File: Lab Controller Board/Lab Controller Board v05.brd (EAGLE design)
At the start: 50 x 50 mm, 52 parts, among them Q2 NPN - 2N5088, Q3 MOSFET-NCHANNELFQP30N06L, Q4 NPN - 2N5088, Q5 MOSFET-NCHANNELFQP30N06L, Q6 NPN - 2N5088, Q7 MOSFET-NCHANNELFQP30N06L, Q8 NPN - 2N5088, U1 ATMEGA328P_TQFP, U2 CH340G, Y1 16MHZ

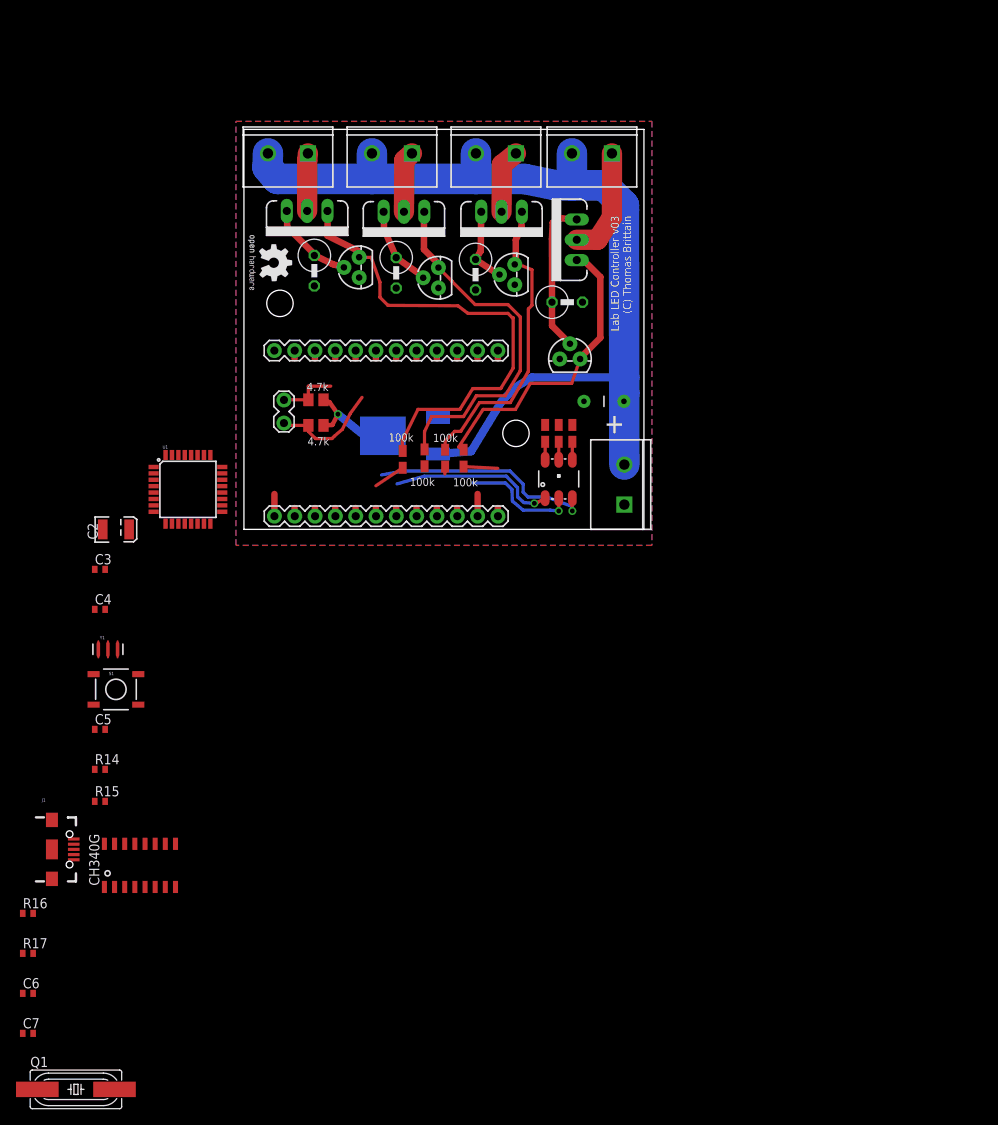
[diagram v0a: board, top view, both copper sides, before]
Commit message: Working on Lab LED
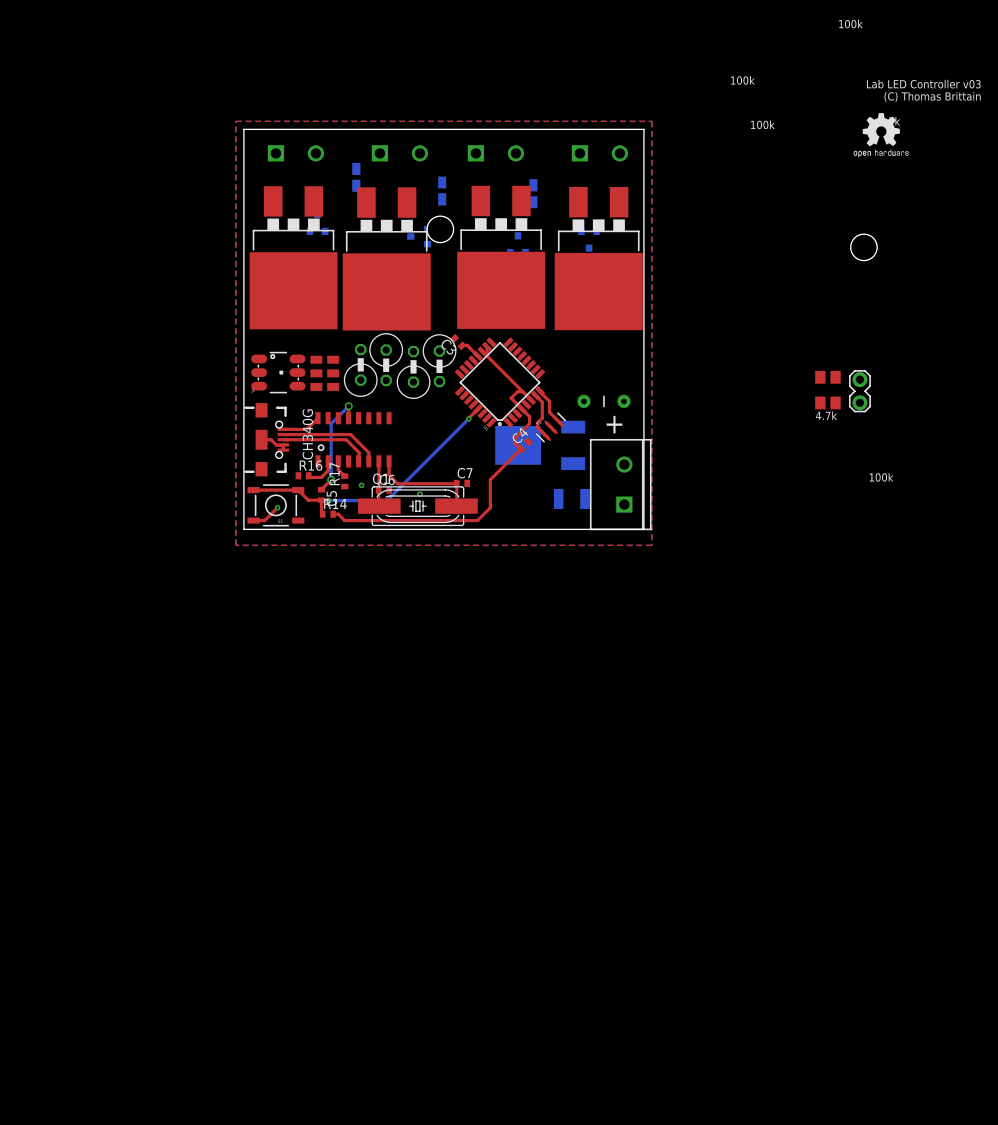
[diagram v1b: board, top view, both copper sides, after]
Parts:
- removed JP6, JP7: (no value), SparkFun-Connectors:1X12
- removed R15: 330, resistor:R0402
- FQP30N06L, Q3, Q5, Q7: value MOSFET-NCHANNELFQP30N06L -> 100A/100V; device SparkFun-DiscreteSemi:TO220V -> SparkFun-DiscreteSemi:TO-263/D2PAK
- Q2, Q4, Q6, Q8: value NPN - 2N5088 -> MMBT5088; device SparkFun-DiscreteSemi:TO-92 -> SparkFun-DiscreteSemi:SOT23-3
- moved C7 87.6 mm to (27.2, 5.75)
- moved Q1 84.5 mm to (21.8, 2.90)
- moved C6 77.0 mm to (17.5, 4.90)
- moved GOLD_ORB_SM2 76.8 mm to (75.8, 45.5), turned to 0 degrees
- moved STANDOFF1 73.3 mm to (77.5, 35.2)
- moved JP8 72.0 mm to (77.0, 16.0), turned to 90 degrees
- moved R17 71.1 mm to (12.6, 6.00), turned to 90 degrees
- moved R16 64.6 mm to (7.45, 6.70)
- moved R9 64.3 mm to (73.0, 19.0), turned to 180 degrees
- moved R10 64.0 mm to (73.0, 15.8), turned to 180 degrees
- moved Y1 62.0 mm to (38.4, 12.7), turned to 45 degrees
- moved U2 59.5 mm to (13.7, 11.2)
- moved GOLD_ORB_SM1 58.2 mm to (106.8, 13.8)
- moved J1 57.5 mm to (2.20, 11.2)
- moved C2 57.1 mm to (41.0, 3.80), flipped to the bottom
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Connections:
- removed net N$10: JP6.3, LED1.2
- removed net N$14: R15.2, U1.17
- removed net N$15: JP7.1
- removed net N$16: JP7.2
- removed net N$17: JP7.3
- removed net N$18: JP7.4
- removed net N$19: JP7.5
- removed net N$20: JP7.6
- removed net N$21: JP7.7
- removed net N$22: JP7.8
- removed net N$23: JP7.9
- removed net N$24: JP7.10
- removed net N$25: JP7.11
- removed net N$26: JP7.12
- removed net N$3: JP6.10
- removed net N$30: U2.10, U2.11, U2.12, U2.14, U2.15, U2.9
- removed net N$4: JP6.9
- removed net RX: JP6.11
- removed net TX: JP6.12
- new net 0: U1.30
- new net 1: U1.31
- new net 10: U1.14
- new net 11: U1.15
- new net 12: U1.16
- new net 13: LED1.2, U1.17
- new net 2: U1.32
- new net 3: U1.1
- new net 4: U1.2
- new net 5: U1.9
- new net 6: U1.10
- new net 7: U1.11
- new net 8: U1.12
- new net A0: U1.23
- new net A1: U1.24
- new net A2: U1.25
- new net A3: U1.26
- new net A4: U1.27
- new net A5: U1.28
- new net A6: U1.19
- new net A7: U1.22
- new net X0: C7.1, Q1.2, U2.8
- new net X1: C6.1, Q1.1, U2.7
- net 9: now also U1.13; no longer JP6.2
- net APM_PIN_3: no longer JP6.7
- net APM_PIN_5: no longer JP6.5
- net APM_PIN_6: no longer JP6.4
- net APM_PIN_9: no longer JP6.1
- net FET_SOURCE: now also Q2.1; no longer Q2.2
- net FET_SOURCE1: now also Q4.1; no longer Q4.2
- net FET_SOURCE2: now also Q6.1; no longer Q6.2
- net FET_SOURCE3: now also Q8.1; no longer Q8.2
- net GND: now also Q2.2, Q4.2, Q6.2, Q8.2; no longer Q2.1, Q4.1, Q6.1, Q8.1
- net N$32: no longer C6.1, C7.1, Q1.1, Q1.2, U2.7, U2.8
- net N$5: no longer JP6.8
- net N$7: no longer JP6.6
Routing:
- net 12V: track 120.1 -> 0.00 mm
- net PWM_B1: track 59.4 -> 0.00 mm
- net VCC: track 0.00 -> 48.6 mm
- net PWM_B: track 45.9 -> 0.00 mm
- net PWM_B2: track 39.4 -> 0.00 mm
- net PWM_B3: track 38.2 -> 0.00 mm
- net N$13: track 0.00 -> 35.2 mm, vias 0 -> 2
- net N$5: track 29.2 -> 0.00 mm, vias 1 -> 0
- net N$7: track 21.9 -> 0.00 mm, vias 1 -> 0
- net FET_SOURCE2: track 19.2 -> 0.00 mm
- net N$10: track 15.5 -> 0.00 mm, vias 1 -> 0
- net LED_DRAIN2: track 13.9 -> 0.00 mm
- net SDA: track 13.7 -> 0.00 mm
- net X0: track 0.00 -> 13.5 mm
- net DTR: track 0.00 -> 13.4 mm, vias 0 -> 2
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
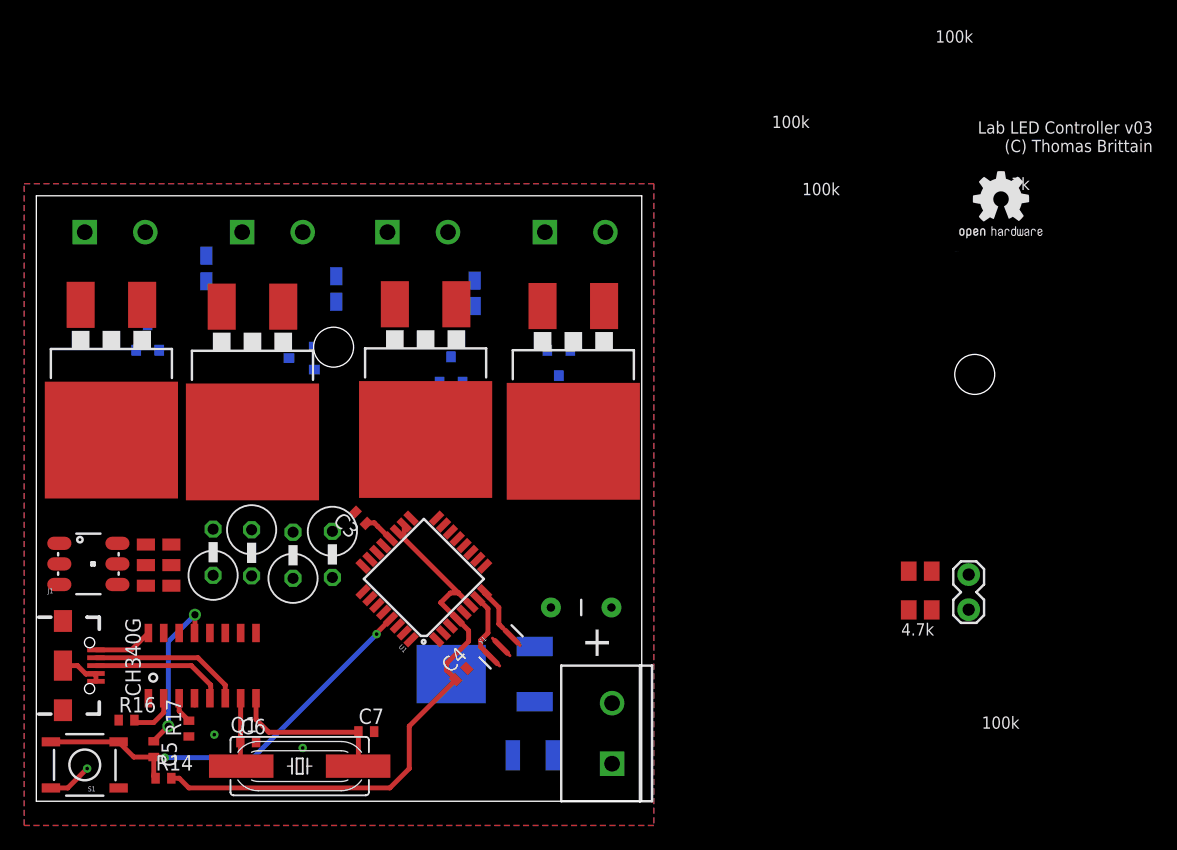
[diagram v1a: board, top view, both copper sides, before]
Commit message: Working
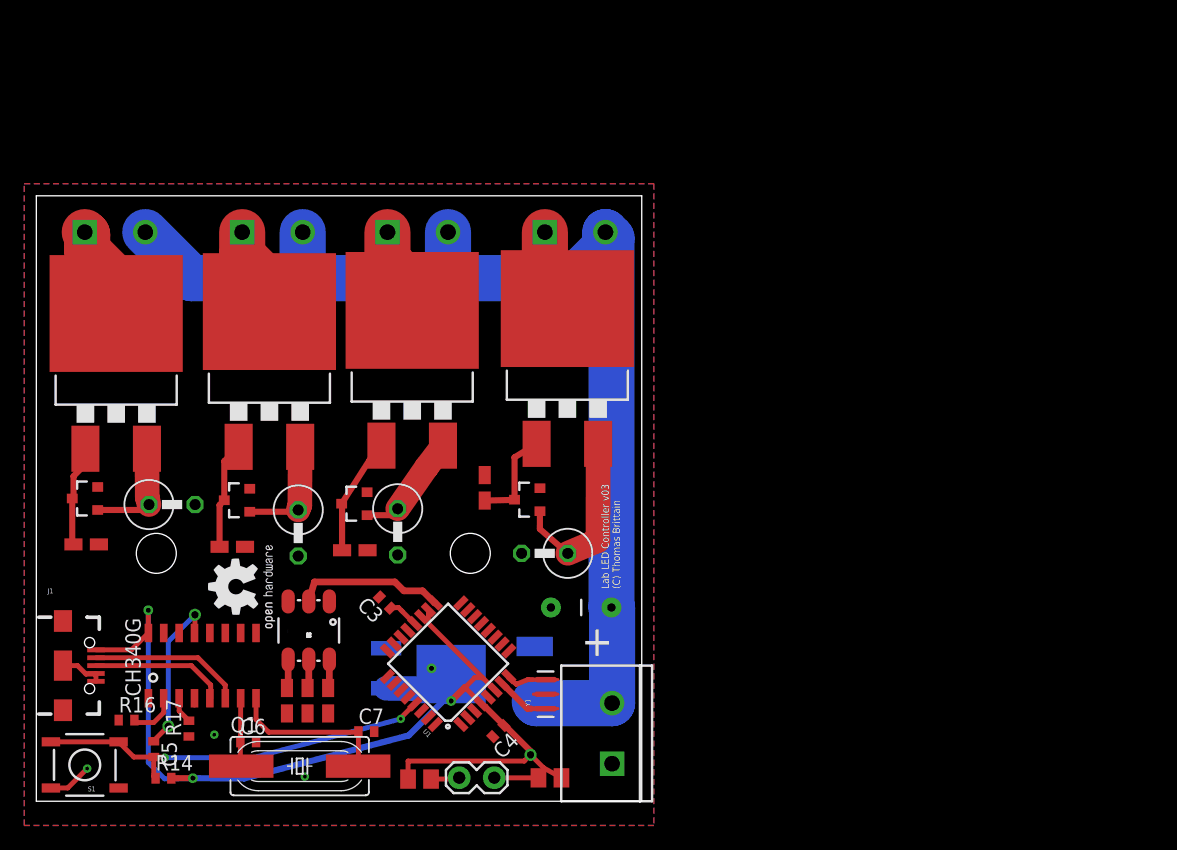
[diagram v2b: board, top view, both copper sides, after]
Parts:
- moved GOLD_ORB_SM1 65.9 mm to (42.8, 29.7)
- moved GOLD_ORB_SM2 63.5 mm to (20.8, 13.9), turned to 90 degrees
- moved STANDOFF1 44.2 mm to (35.8, 20.5)
- moved JP8 44.2 mm to (35.1, 1.94), turned to 0 degrees
- moved R10 43.6 mm to (31.6, 1.83)
- moved R9 35.0 mm to (42.4, 1.93), turned to 0 degrees
- moved R3 24.9 mm to (4.12, 21.2), flipped to the top, turned to 180 degrees
- moved R7 23.4 mm to (26.3, 20.7), flipped to the top, turned to 180 degrees
- moved R1 23.0 mm to (16.2, 21.0), flipped to the top, turned to 180 degrees
- moved STANDOFF2 22.5 mm to (9.91, 20.5)
- moved R12 19.0 mm to (24.1, 8.30), turned to 90 degrees
- moved LED1 19.0 mm to (22.5, 14.1), turned to 270 degrees
- moved R6 16.9 mm to (41.3, 20.5), turned to 180 degrees
- moved R13 16.6 mm to (22.4, 8.30), turned to 90 degrees
- moved R11 14.2 mm to (20.7, 8.30), turned to 90 degrees
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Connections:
- removed net 5V: J1.VBUS, R10.2, R9.2, U2.16
- net VCC: now also J1.VBUS, R10.2, R9.2, U2.16
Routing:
- net 12V: track 0.00 -> 95.6 mm
- net VCC: track 48.6 -> 92.4 mm, vias 0 -> 4
- net FET_SOURCE2: track 0.00 -> 15.2 mm
- net 13: track 0.00 -> 12.4 mm
- net PWM_B3: track 0.00 -> 9.68 mm
- net FET_SOURCE: track 0.00 -> 9.28 mm
- net FET_SOURCE3: track 0.00 -> 9.21 mm
- net FET_SOURCE1: track 0.00 -> 9.16 mm
- net PWM_B: track 0.00 -> 8.91 mm
- net PWM_B1: track 0.00 -> 8.65 mm
- net PWM_B2: track 0.00 -> 8.10 mm
- net LED_DRAIN1: track 0.00 -> 8.00 mm
- net LED_DRAIN3: track 0.00 -> 7.53 mm
- net LED_DRAIN: track 0.00 -> 7.49 mm
- net LED_DRAIN2: track 0.00 -> 6.94 mm
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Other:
- board text added: "Lab LED Controller v05 (C) Thomas Brittain"
- board text removed: "100k"
- board text removed: "4.7k"
- board text removed: "MC7805CD2TR4"

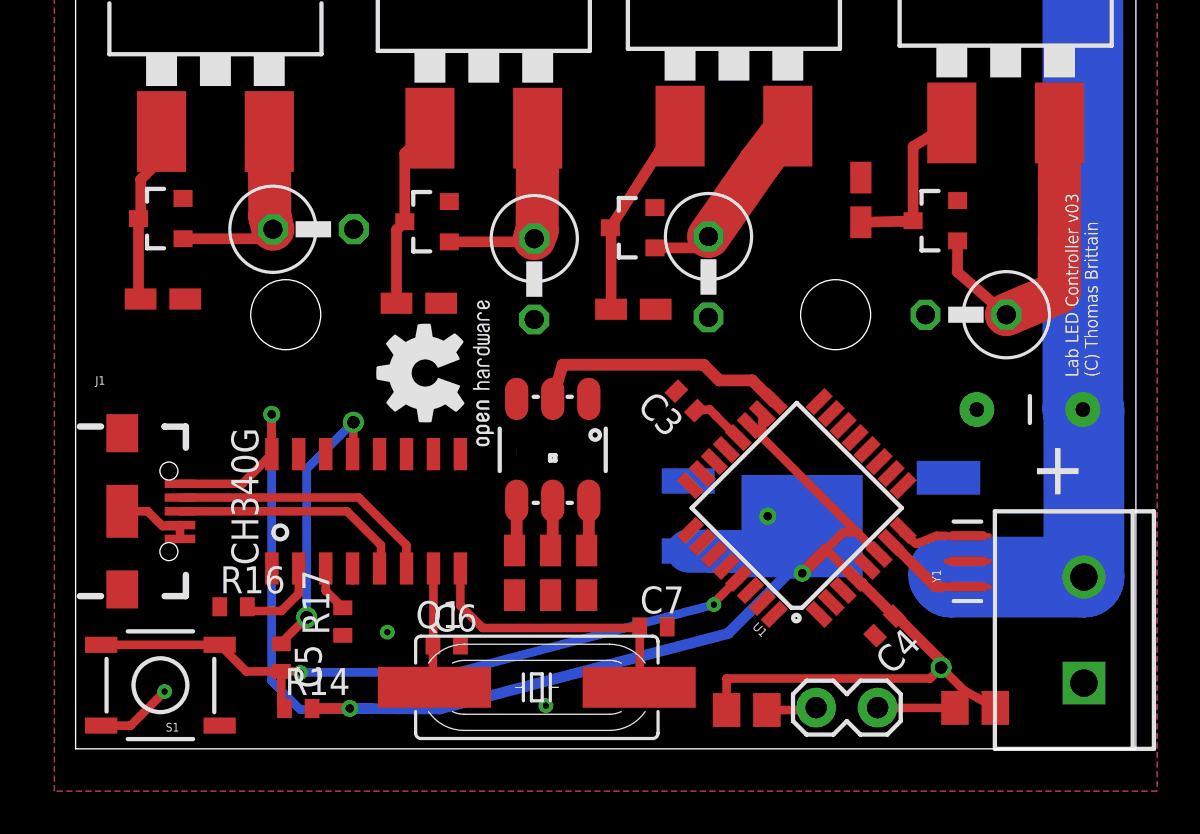
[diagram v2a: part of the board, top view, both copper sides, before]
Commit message: Lab Controller
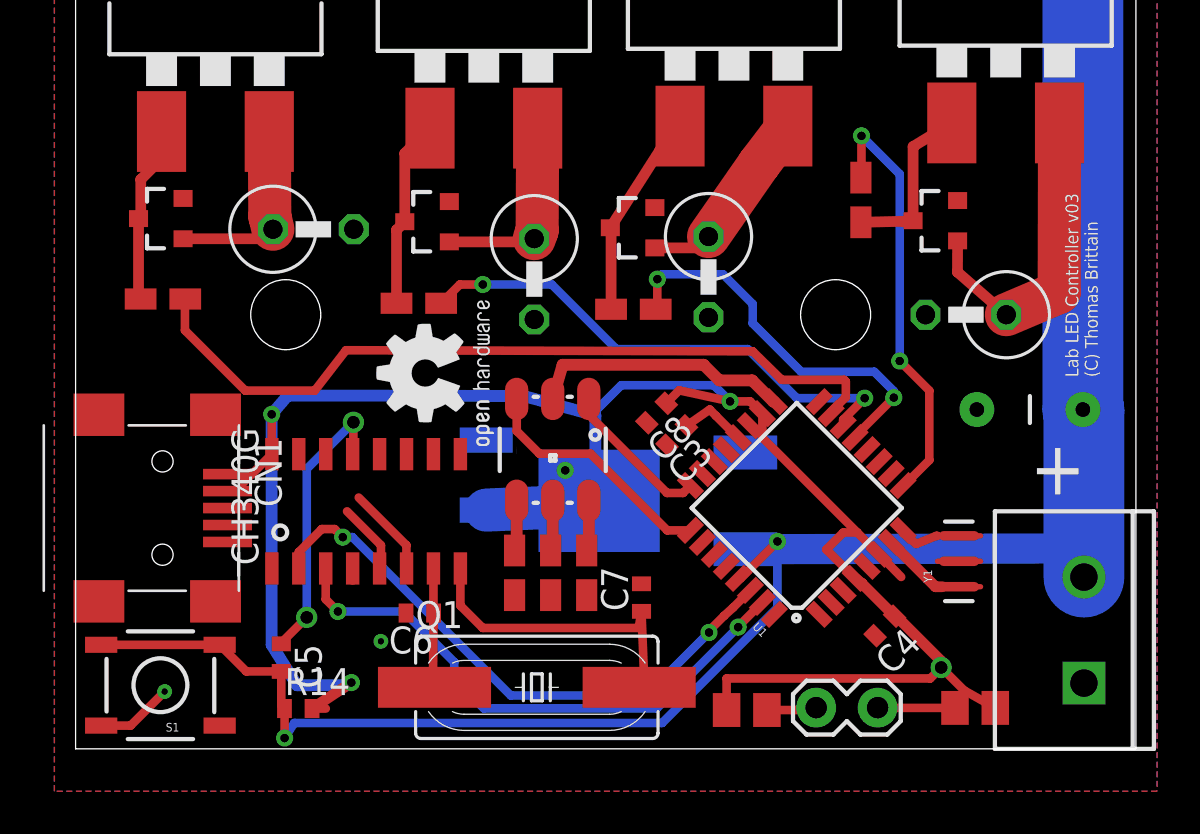
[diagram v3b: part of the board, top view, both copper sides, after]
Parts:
- removed J1: (no value), SparkFun-Connectors:USB-B-MICRO-SMD_V03
- removed R16, R17: 1k, resistor:R0402
- added C8: 0.1uF, resistor:C0402
- added CN1: (no value), adafruit:USB-MINIB
- moved C2 9.72 mm to (19.4, 12.9)
- moved MC7805CD2TR4 9.65 mm to (26.3, 11.7)
- moved C6 1.97 mm to (16.2, 6.40), turned to 180 degrees
- moved C3 1.69 mm to (28.3, 14.8), turned to 225 degrees
- moved C7 1.49 mm to (26.7, 7.13), turned to 90 degrees
- moved Y1 0.41 mm to (41.7, 8.84)
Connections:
- removed net 0: U1.30
- removed net 1: U1.31
- removed net APM_PIN_3: R3.1
- removed net APM_PIN_5: R1.1
- removed net APM_PIN_6: R7.1
- removed net APM_PIN_9: R5.1
- removed net N$5: LED1.3
- removed net N$7: LED1.1
- new net ID: CN1.ID
- net 10: now also R1.1
- net 11: now also R3.1
- net 5: now also R5.1
- net 9: now also R7.1
- net A1: now also LED1.1
- net A2: now also LED1.3
- net D+: now also CN1.D+; no longer J1.D+
- net D-: now also CN1.D-; no longer J1.D-
- net GND: now also C8.2, CN1.GND; no longer J1.GND, J1.ID, J1.SHIELD1, J1.SHIELD2, J1.SHIELD3
- net U2_RX: now also U1.31; no longer R17.2
- net U2_TX: now also U1.30; no longer R16.2
- net VCC: now also C8.1, CN1.VBUS; no longer J1.VBUS
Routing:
- net 11: track 0.00 -> 37.1 mm
- net U2_RX: track 2.19 -> 26.7 mm, vias 0 -> 2
- net 10: track 0.00 -> 24.3 mm, vias 0 -> 2
- net U2_TX: track 4.03 -> 27.9 mm, vias 0 -> 2
- net 5: track 0.00 -> 20.3 mm, vias 0 -> 2
- net 9: track 0.00 -> 18.5 mm, vias 0 -> 2
- net A2: track 0.00 -> 11.6 mm
- net N$13: track 33.4 -> 43.8 mm
- net 12V: track 95.6 -> 105.8 mm
- net D-: track 12.7 -> 4.28 mm
- net D+: track 11.3 -> 3.38 mm
- net A1: track 0.00 -> 7.21 mm
- net VCC: track 92.4 -> 96.2 mm
- net GND: track 7.34 -> 3.66 mm, vias 4 -> 3
- net X0: track 13.5 -> 15.3 mm
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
